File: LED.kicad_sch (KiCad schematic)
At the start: 15 parts, among them IC1 MAX25603AUI_V+

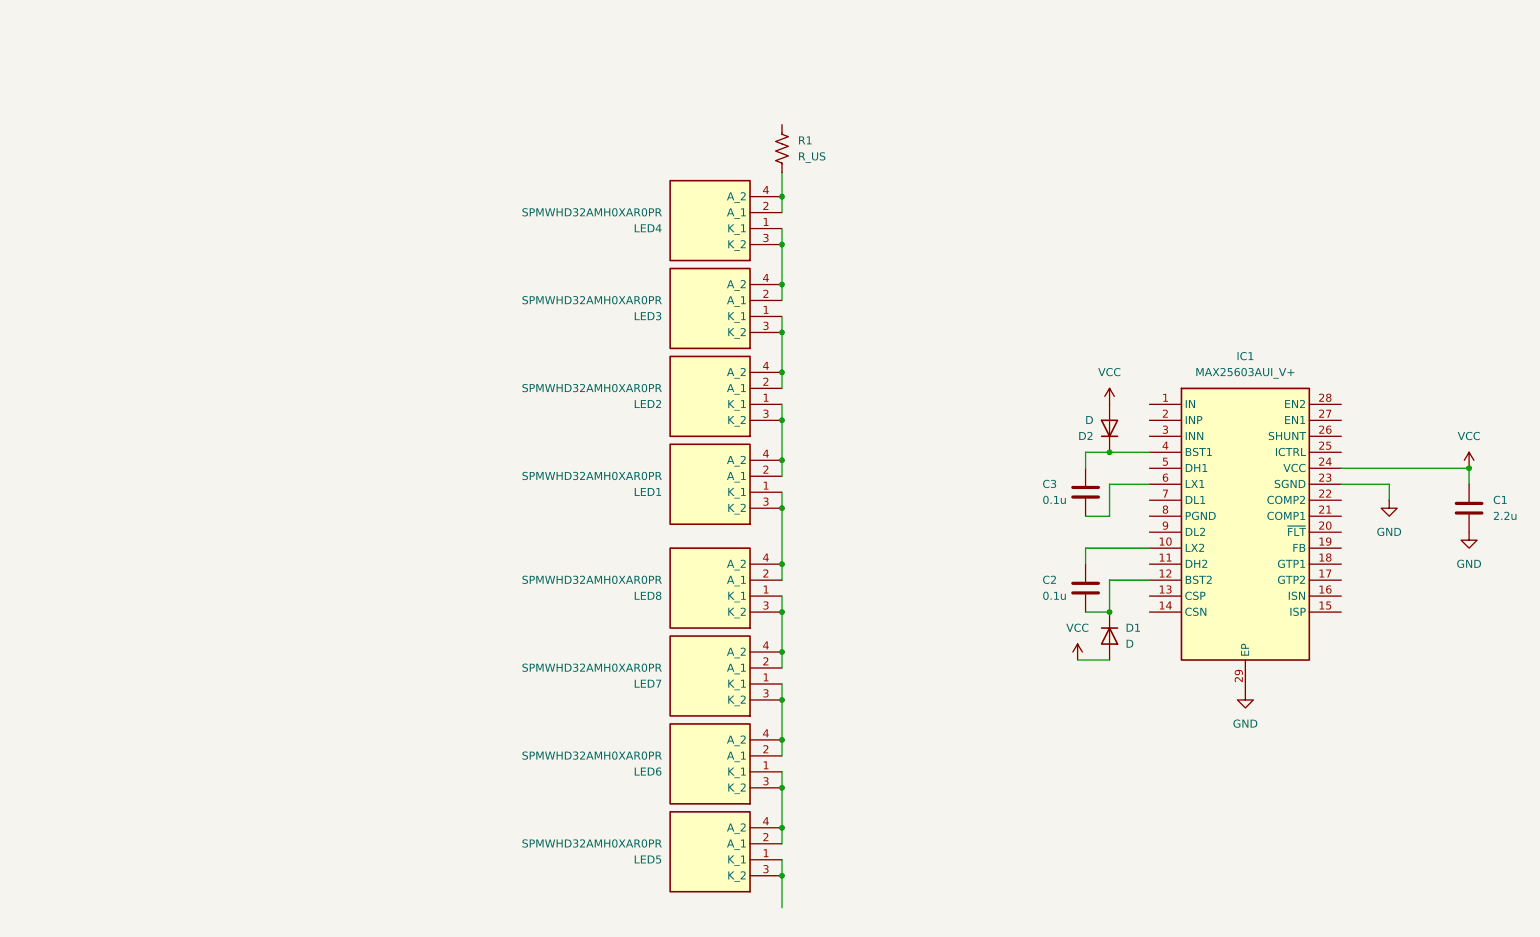
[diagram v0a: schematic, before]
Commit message: Update LED.kicad_sch
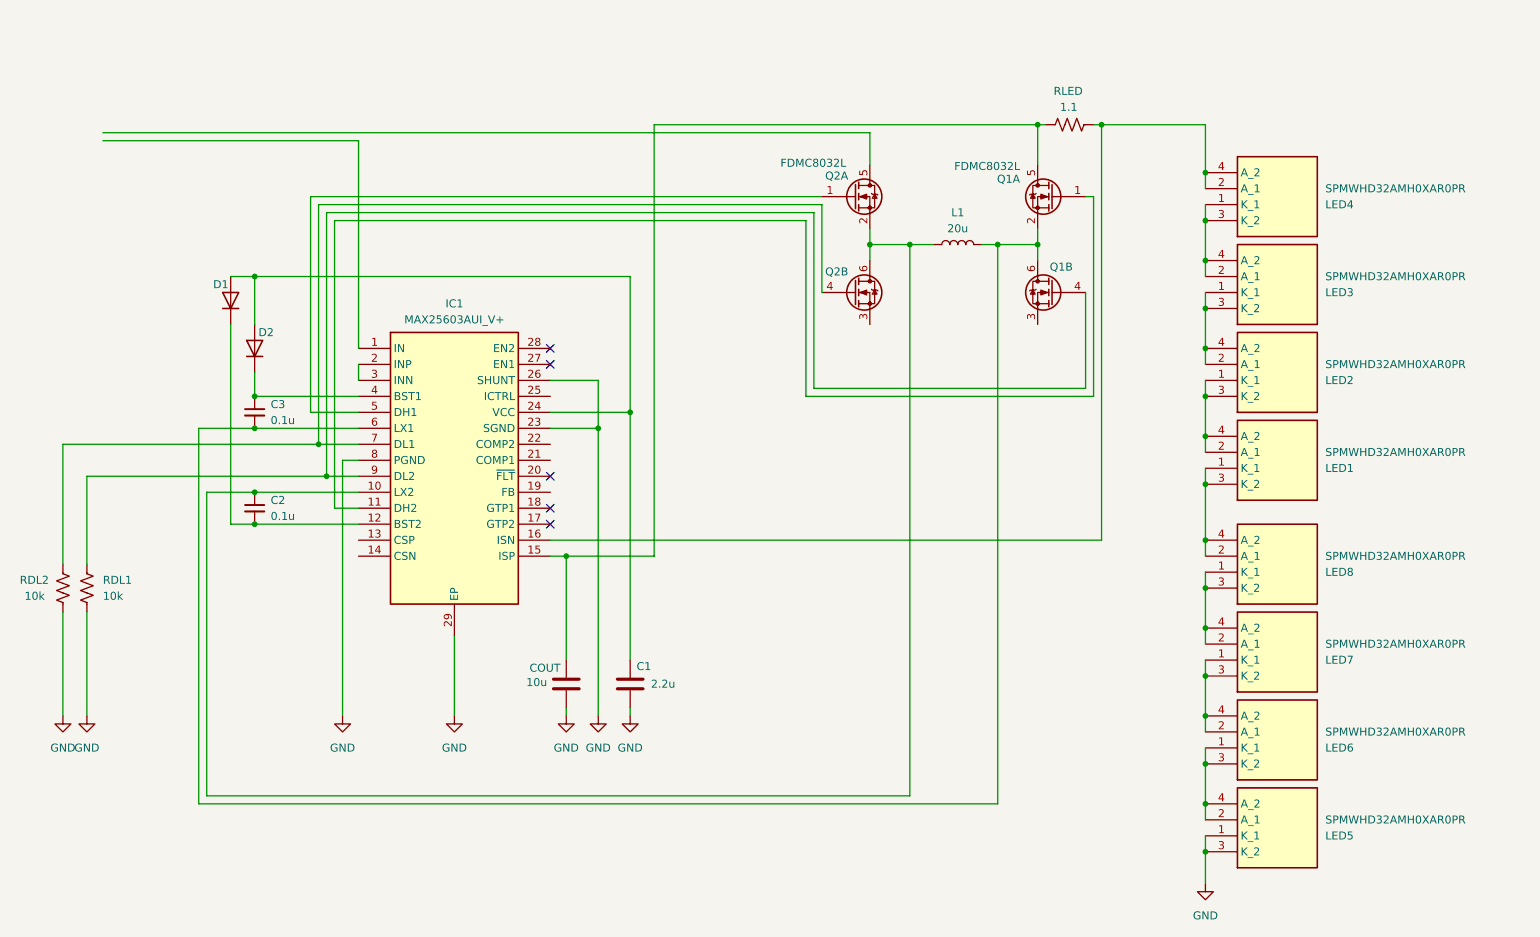
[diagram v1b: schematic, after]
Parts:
- removed C2, C3: 0.1u, 3rdparty:CAPC2012X140N, symbol Device:C
- removed R1: R_US, symbol Device:R_US
- added C2, C3: 0.1u, symbol Device:C_Small
- added COUT: 10u, 3rdparty:CAPC2012X140N, symbol Device:C
- added L1: 20u, symbol Device:L
- added Q1, Q2: FDMC8032L, Package_SON:Fairchild_DualPower33-6_3x3mm, symbol Transistor_FET:FDMC8032L
- added RDL1, RDL2: 10k, symbol Device:R_US
- added RLED: 1.1, symbol Device:R_US
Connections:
- net GND: now also IC1.26 (SHUNT), IC1.8 (PGND), LED5.1 (K_1), LED5.3 (K_2), COUT.2, RDL1.2, RDL2.2
- net at LED4.2 (A_1), LED4.4 (A_2): now also IC1.16 (ISN), RLED.1
- net at D1.1 (K), IC1.12 (BST2): now also C2.2
- net at IC1.10 (LX2): now also C2.1, L1.1, Q2.2 (S1), Q2.6 (D2)
- net at IC1.11 (DH2): now also Q1.1 (G1)
- net at IC1.15 (ISP): now also COUT.1, Q1.5 (D1), RLED.2
- net at IC1.2 (INP): now also IC1.3 (INN)
- net at D2.1 (K), IC1.4 (BST1): now also C3.1
- net at IC1.5 (DH1): now also Q2.1 (G1)
- net at IC1.6 (LX1): now also C3.2, L1.2, Q1.2 (S1), Q1.6 (D2)
- net at IC1.7 (DL1): now also Q2.4 (G2), RDL2.1
- net at IC1.9 (DL2): now also Q1.4 (G2), RDL1.1
- net VCC: no longer names the net of C1.1, D1.2 (A), D2.2 (A), IC1.24 (VCC)
- no-connect marks 0 -> 5
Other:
- moved on the sheet: C1, IC1, LED1, LED2, LED3, LED4, LED5, LED6, LED7, LED8

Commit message: working for free
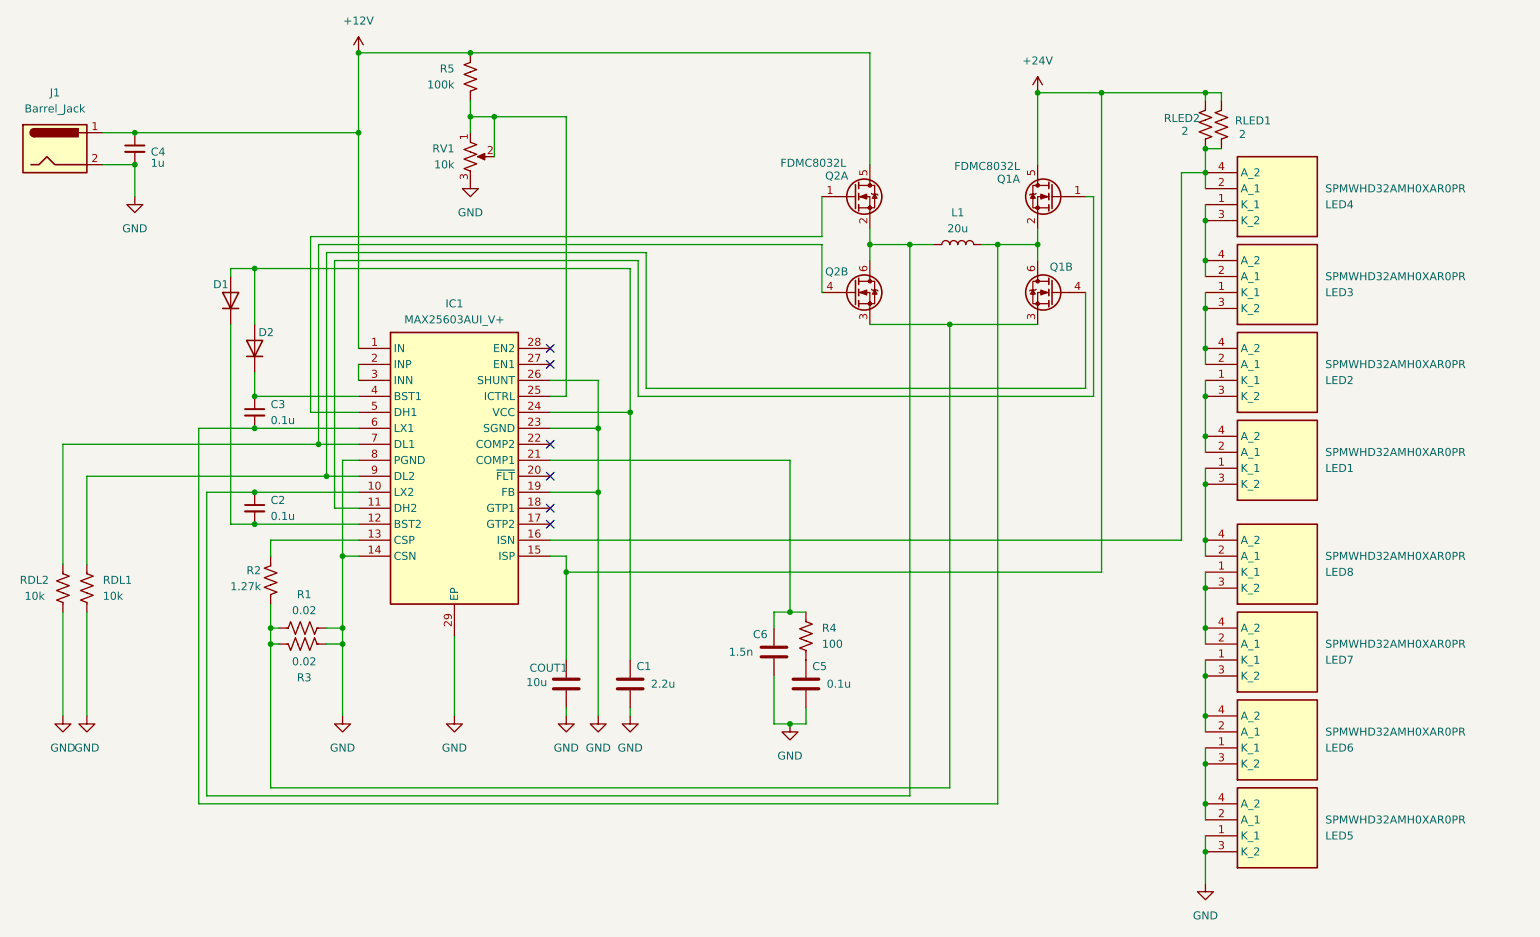
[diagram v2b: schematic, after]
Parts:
- added C4: 1u, symbol Device:C_Small
- added C5: 0.1u, 3rdparty:CAPC2012X140N, symbol Device:C
- added C6: 1.5n, 3rdparty:CAPC2012X140N, symbol Device:C
- added J1: Barrel_Jack, symbol Connector:Barrel_Jack
- added R1, R3: 0.02, symbol Device:R_US
- added R2: 1.27k, symbol Device:R_US
- added R4: 100, symbol Device:R_US
- added R5: 100k, symbol Device:R_US
- added RLED1: 2, symbol Device:R_US
- added RV1: 10k, symbol Device:R_Potentiometer_US
- RLED2: renamed from RLED; value 1.1 -> 2
- renumbered COUT to COUT1
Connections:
- net GND: now also IC1.14 (CSN), IC1.19 (FB), C4.2, C5.2, C6.2, J1.2, R1.1, R3.1, RV1.3
- net at Q2.3 (S2): now also Q1.3 (S2), R1.2, R2.2, R3.2
- net +24V: now reaches COUT1.1, IC1.15 (ISP), Q1.5 (D1), RLED2.2
- net +24V: now also RLED1.2
- net at IC1.16 (ISN), LED4.2 (A_1), LED4.4 (A_2)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: now also RLED1.1
- net +12V: now reaches IC1.1 (IN)
- net +12V: now also Q2.5 (D1), C4.1, J1.1, R5.1
- net at IC1.13 (CSP): now also R2.1
- net at IC1.21 (COMP1): now also C6.1, R4.1
- net at IC1.25 (ICTRL): now also R5.2, RV1.1, RV1.2
- new net: C5.1, R4.2
- no-connect marks 5 -> 6
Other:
- moved on the sheet: RLED2

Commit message: placed leds
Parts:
- D1, D2: footprint Package_TO_SOT_SMD:TO-252-2 -> Diode_SMD:D_SOD-123
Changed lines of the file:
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@@
 			)
 		)
-		(property "Footprint" "Package_TO_SOT_SMD:TO-252-2"
+		(property "Footprint" "Diode_SMD:D_SOD-123"
 			(at 50.8 59.69 0)
 			(effects
@@
 			)
 		)
-		(property "Footprint" "Package_TO_SOT_SMD:TO-252-2"
+		(property "Footprint" "Diode_SMD:D_SOD-123"
 			(at 54.61 67.31 0)
 			(effects

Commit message: more free work (done pcb)
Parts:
- C2, C3, C4: footprint (none) -> Capacitor_SMD:CAPC2012X140N
- IC1: footprint SOP65P640X110-29N -> LED_SMD:SOP65P640X110-29N
- J1: footprint (none) -> Connector_BarrelJack:BarrelJack_Horizontal
- L1: footprint (none) -> Inductor_SMD_Wurth:7843332000
- LED1, LED2, LED3, LED4, LED5, LED6, LED7, LED8: footprint SPMWHD32AMH0XAR0PR -> LED_SMD:SPMWHD32AMH0XAR0PR
- R1, R2, R3, R4, R5, RDL1, RDL2, RLED1, RLED2: footprint (none) -> Resistor_SMD:R_0805_2012Metric
- RV1: footprint (none) -> Potentiometer_SMD:Potentiometer_Vishay_TS53YJ_Vertical
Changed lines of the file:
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@@
 			)
 		)
-		(property "Footprint" ""
+		(property "Footprint" "Resistor_SMD:R_0805_2012Metric"
 			(at 87.884 24.384 90)
 			(effects
@@
 			)
 		)
-		(property "Footprint" ""
+		(property "Footprint" "Connector_BarrelJack:BarrelJack_Horizontal"
 			(at 24.13 36.576 0)
 			(effects
@@
 			)
 		)
-		(property "Footprint" ""
+		(property "Footprint" "Resistor_SMD:R_0805_2012Metric"
 			(at 143.256 113.284 90)
 			(effects
@@
 			)
 		)
-		(property "Footprint" ""
+		(property "Footprint" "Capacitor_SMD:CAPC2012X140N"
 			(at 54.61 77.47 0)
 			(effects
@@
 			)
 		)
-		(property "Footprint" "SPMWHD32AMH0XAR0PR"
+		(property "Footprint" "LED_SMD:SPMWHD32AMH0XAR0PR"
 			(at 224.79 52.4 0)
 			(effects
@@
 			)
 		)
-		(property "Footprint" ""
+		(property "Footprint" "Resistor_SMD:R_0805_2012Metric"
 			(at 56.134 104.394 90)
 			(effects
@@
 			)
 		)
-		(property "Footprint" "SPMWHD32AMH0XAR0PR"
+		(property "Footprint" "LED_SMD:SPMWHD32AMH0XAR0PR"
 			(at 224.79 -6.02 0)
 			(effects
@@
 			)
 		)
-		(property "Footprint" ""
+		(property "Footprint" "Potentiometer_SMD:Potentiometer_Vishay_TS53YJ_Vertical"
 			(at 88.9 36.83 0)
 			(effects
@@
 			)
 		)
-		(property "Footprint" ""
+		(property "Footprint" "Resistor_SMD:R_0805_2012Metric"
 			(at 28.956 105.664 90)
 			(effects
@@
 			)
 		)
-		(property "Footprint" ""
+		(property "Footprint" "Resistor_SMD:R_0805_2012Metric"
 			(at 209.296 31.496 90)
 			(effects
@@
 			)
 		)
-		(property "Footprint" ""
+		(property "Footprint" "Resistor_SMD:R_0805_2012Metric"
 			(at 206.756 31.496 90)
 			(effects
@@
 			)
 		)
-		(property "Footprint" "SPMWHD32AMH0XAR0PR"
+		(property "Footprint" "LED_SMD:SPMWHD32AMH0XAR0PR"
 			(at 224.79 -33.96 0)
 			(effects
@@
 			)
 		)
-		(property "Footprint" "SPMWHD32AMH0XAR0PR"
+		(property "Footprint" "LED_SMD:SPMWHD32AMH0XAR0PR"
 			(at 224.79 -19.99 0)
 			(effects
@@
 			)
 		)
-		(property "Footprint" ""
+		(property "Footprint" "Resistor_SMD:R_0805_2012Metric"
 			(at 61.976 113.284 90)
 			(effects
@@
 			)
 		)
-		(property "Footprint" "SPMWHD32AMH0XAR0PR"
+		(property "Footprint" "LED_SMD:SPMWHD32AMH0XAR0PR"
 			(at 224.79 24.46 0)
 			(effects
@@
 			)
 		)
-		(property "Footprint" ""
+		(property "Footprint" "Resistor_SMD:R_0805_2012Metric"
 			(at 25.146 105.664 90)
 			(effects
@@
 			)
 		)
-		(property "Footprint" ""
+		(property "Footprint" "Resistor_SMD:R_0805_2012Metric"
 			(at 61.976 112.776 90)
 			(effects
@@
 			)
 		)
-		(property "Footprint" ""
+		(property "Footprint" "Capacitor_SMD:CAPC2012X140N"
 			(at 54.61 92.71 0)
 			(effects
@@
 			)
 		)
-		(property "Footprint" ""
+		(property "Footprint" "Inductor_SMD_Wurth:7843332000"
 			(at 166.37 50.8 0)
 			(effects
@@
 			)
 		)
-		(property "Footprint" "SOP65P640X110-29N"
+		(property "Footprint" "LED_SMD:SOP65P640X110-29N"
 			(at 97.79 162.23 0)
 			(effects
@@
 			)
 		)
-		(property "Footprint" "SPMWHD32AMH0XAR0PR"
+		(property "Footprint" "LED_SMD:SPMWHD32AMH0XAR0PR"
 			(at 224.79 -47.93 0)
 			(effects
@@
 			)
 		)
-		(property "Footprint" "SPMWHD32AMH0XAR0PR"
+		(property "Footprint" "LED_SMD:SPMWHD32AMH0XAR0PR"
 			(at 224.79 10.49 0)
 			(effects
@@
 			)
 		)
-		(property "Footprint" ""
+		(property "Footprint" "Capacitor_SMD:CAPC2012X140N"
 			(at 35.56 35.56 0)
 			(effects
@@
 			)
 		)
-		(property "Footprint" "SPMWHD32AMH0XAR0PR"
+		(property "Footprint" "LED_SMD:SPMWHD32AMH0XAR0PR"
 			(at 224.79 38.43 0)
 			(effects
